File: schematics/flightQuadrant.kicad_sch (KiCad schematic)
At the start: 14 parts, among them M1 M_ENG1, M2 M_ENG2, M3 M_BRK, M4 M_FLP, U1 ta7291sgo, U2 ta7291sgo, U3 ta7291sgo, U4 ta7291sgo

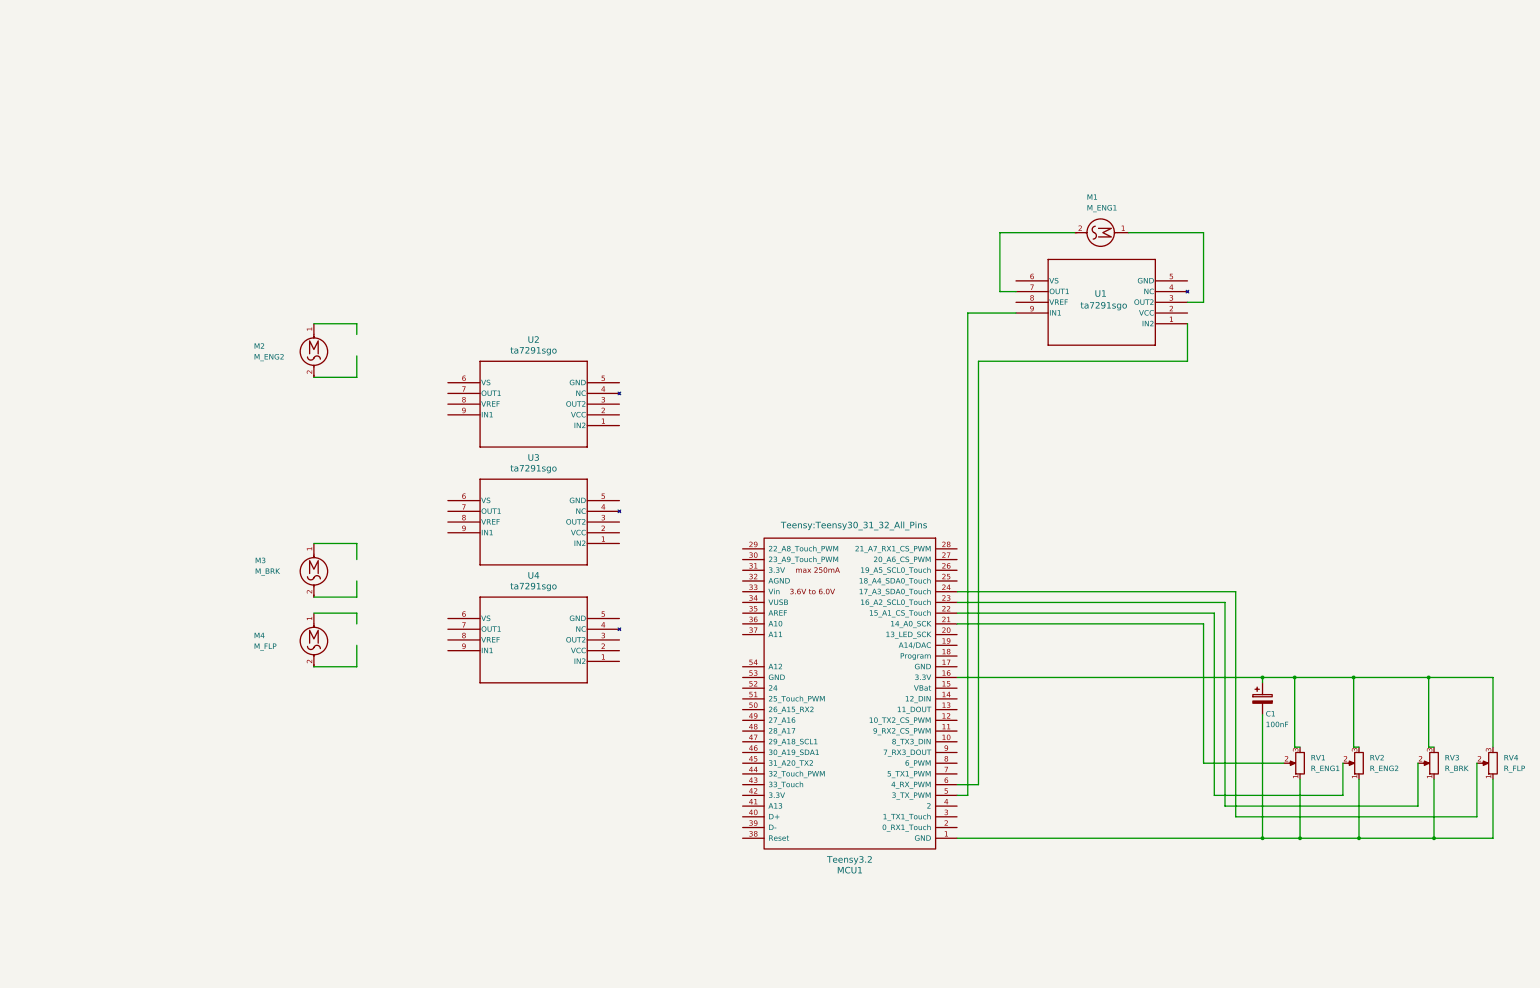
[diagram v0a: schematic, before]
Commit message: Update arduino code firmware!
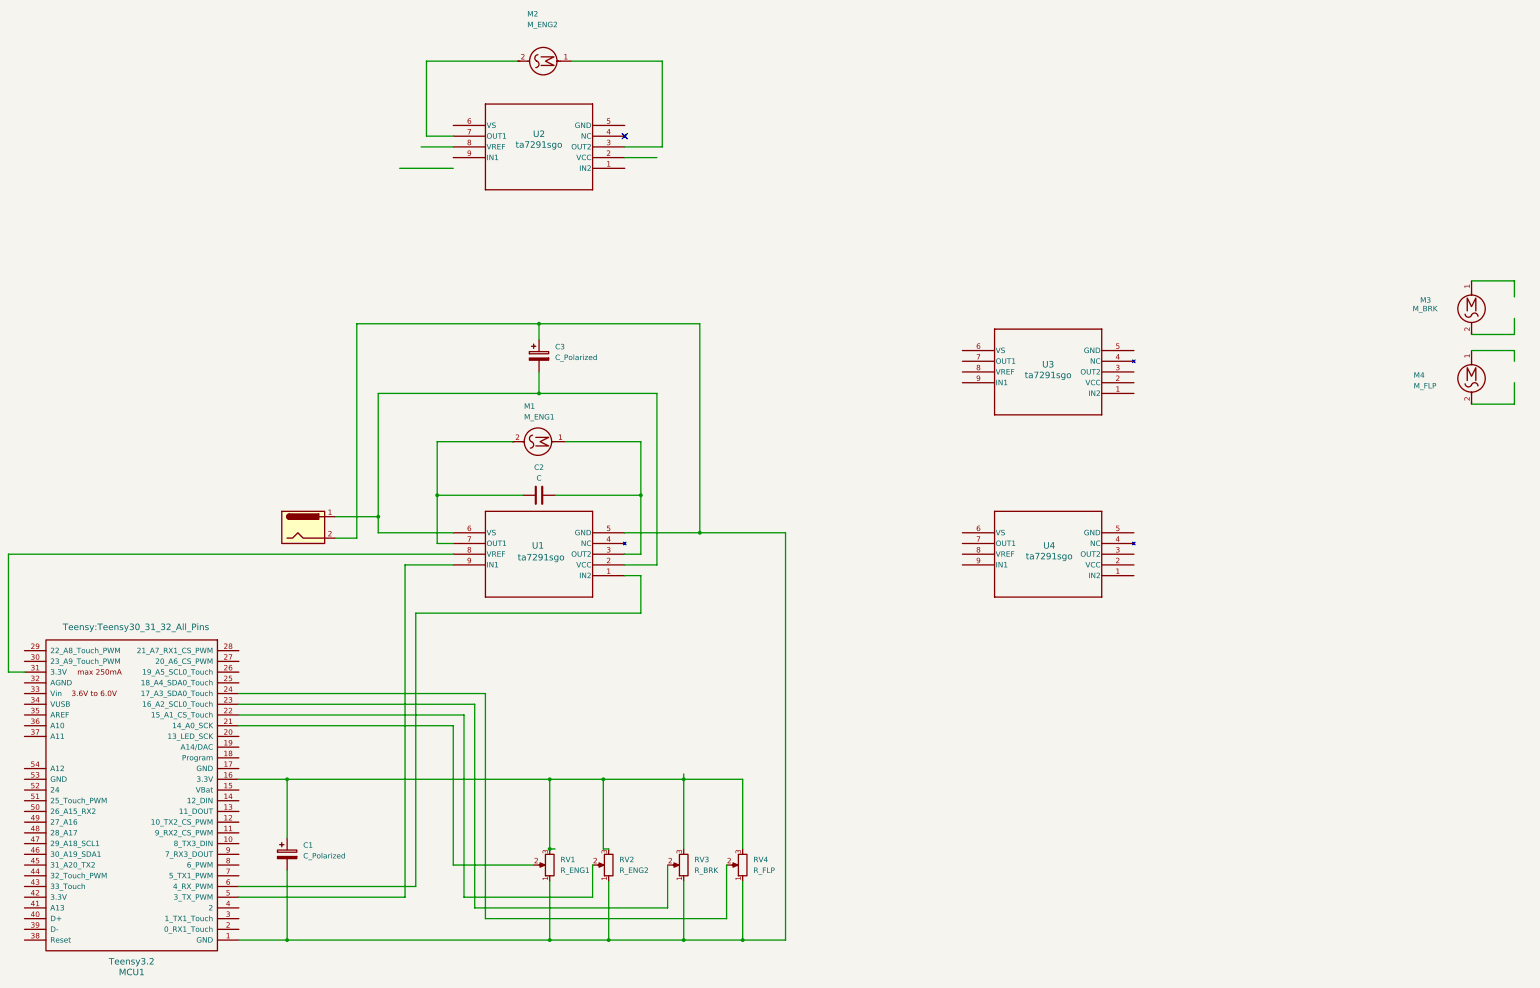
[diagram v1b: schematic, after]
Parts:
- added C2: C, symbol Device:C
- added C3: C_Polarized, symbol Device:C_Polarized
- added J1: Barrel_Jack, symbol Connector:Barrel_Jack
- C1: value 100nF -> C_Polarized; footprint Capacitor_THT:CP_Radial_D5.0mm_P2.00mm -> (none)
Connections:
- net at U1.2 (VCC): now also U1.6 (VS), C3.2, J1.1
- net at M1.1, U1.3 (OUT2): now also C2.2
- net at U1.5 (GND): now also C1.2, MCU1.1 (GND), RV1.1, RV2.1, RV3.1, RV4.1, C3.1, J1.2
- net at M1.2, U1.7 (OUT1): now also C2.1
- net at U1.8 (VREF): now also MCU1.31 (3.3V)
- net at U2.3 (OUT2): now also M2.1
- net at U2.7 (OUT1): now also M2.2
- no-connect marks 0 -> 1
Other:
- moved on the sheet: M1, M2, M3, M4, MCU1, RV1, RV2, RV3, RV4, U1, U2, U3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
